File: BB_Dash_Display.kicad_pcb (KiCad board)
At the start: 2 copper layers, 54.6 x 61 mm, 47 parts, among them J1 FH12-40S-0.5SH, J2 Mini_SPOX, J3 Mini_SPOX, P8 BeagleBone_Black_Header, P9 BeagleBone_Black_Header, U1 TPS61165, U2 TCAN1042V, U3 TPS562200

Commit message: archive stuff
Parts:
- C1, C10, C11, C4, C5, C6, C7: footprint Capacitor_SMD:C_0805_2012Metric -> archive:C_0805_2012Metric
- C2, C8, C9: footprint Capacitor_SMD:C_1206_3216Metric -> archive:C_1206_3216Metric
- C3: footprint Capacitor_SMD:C_1210_3225Metric -> archive:C_1210_3225Metric
- D1, D2: footprint Diode_SMD:D_SOD-123 -> archive:D_SOD-123
- F1: footprint Fuse:Fuseholder_Littelfuse_Nano2_154x -> archive:Fuseholder_Littelfuse_Nano2_154x
- G***: footprint project:OUR-Logo -> archive:OUR-Logo
- J1: footprint Connector_FFC-FPC:Hirose_FH12-40S-0.5SH_1x40-1MP_P0.50mm_Horizontal -> archive:Hirose_FH12-40S-0.5SH_1x40-1MP_P0.50mm_Horizontal
- J2: footprint Connector_Molex:Molex_SPOX_5268-03A_1x03_P2.50mm_Horizontal -> archive:Molex_SPOX_5268-03A_1x03_P2.50mm_Horizontal
- J3: footprint Connector_Molex:Molex_SPOX_5268-02A_1x02_P2.50mm_Horizontal -> archive:Molex_SPOX_5268-02A_1x02_P2.50mm_Horizontal
- JP1: footprint Jumper:SolderJumper-2_P1.3mm_Open_TrianglePad1.0x1.5mm -> archive:SolderJumper-2_P1.3mm_Open_TrianglePad1.0x1.5mm
- L1, L2: footprint Inductor_SMD:L_Bourns-SRN4018 -> archive:L_Bourns-SRN4018
- P8, P9: footprint project:PinHeader_2x23_P2.54mm_Vertical_Flip -> archive:PinHeader_2x23_P2.54mm_Vertical_Flip
- R1, R2, R3, R4, R5, R6: footprint Resistor_SMD:R_0805_2012Metric -> archive:R_0805_2012Metric
- REF**: footprint project:BeagleBone-Black_Flip -> archive:BeagleBone-Black_Flip
- RN1, RN2, RN3, RN4, RN5: footprint Resistor_SMD:R_Array_Convex_4x0603 -> archive:R_Array_Convex_4x0603
- TP1, TP2, TP3, TP4, TP5, TP6, TP7, TP8, TP9: footprint TestPoint:TestPoint_THTPad_D2.0mm_Drill1.0mm -> archive:TestPoint_THTPad_D2.0mm_Drill1.0mm
- U1, U3: footprint Package_TO_SOT_SMD:SOT-23-6 -> archive:SOT-23-6
- U2: footprint Package_SO:SOIC-8_3.9x4.9mm_P1.27mm -> archive:SOIC-8_3.9x4.9mm_P1.27mm

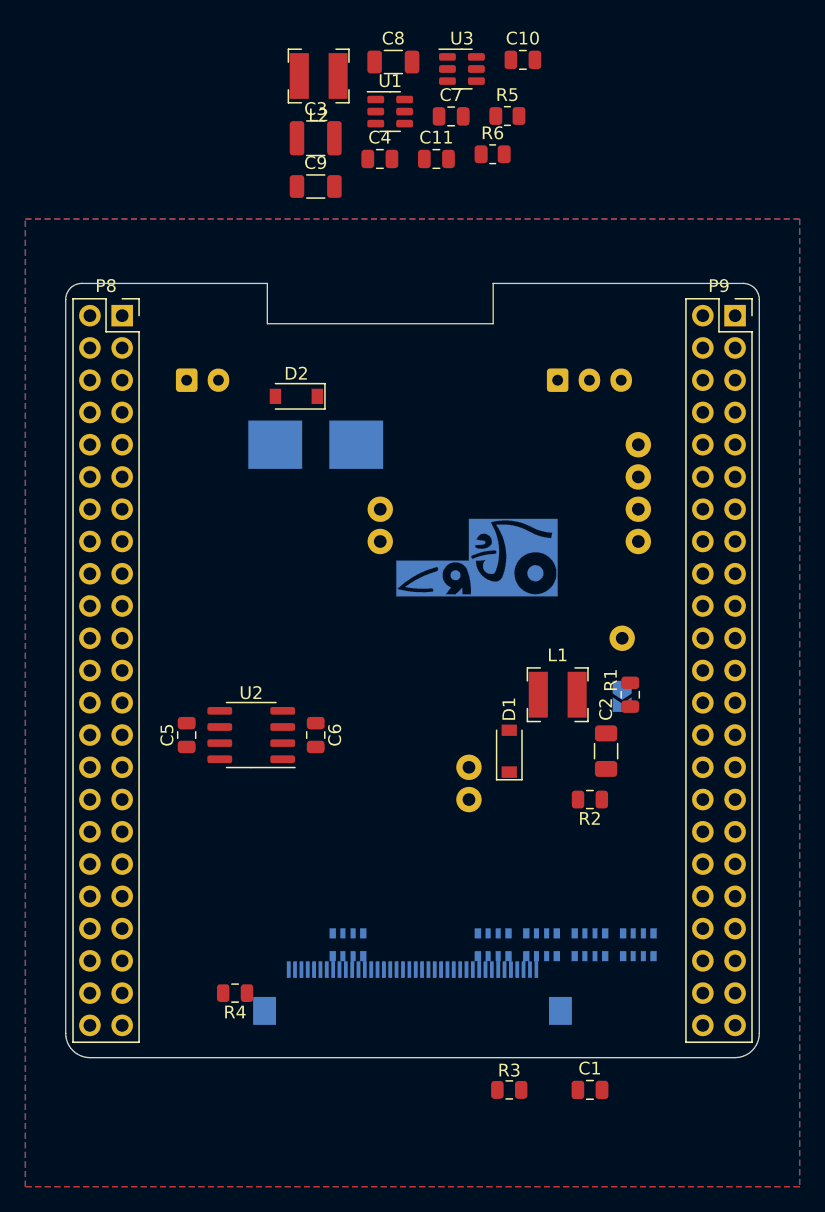
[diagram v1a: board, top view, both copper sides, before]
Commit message: rev b
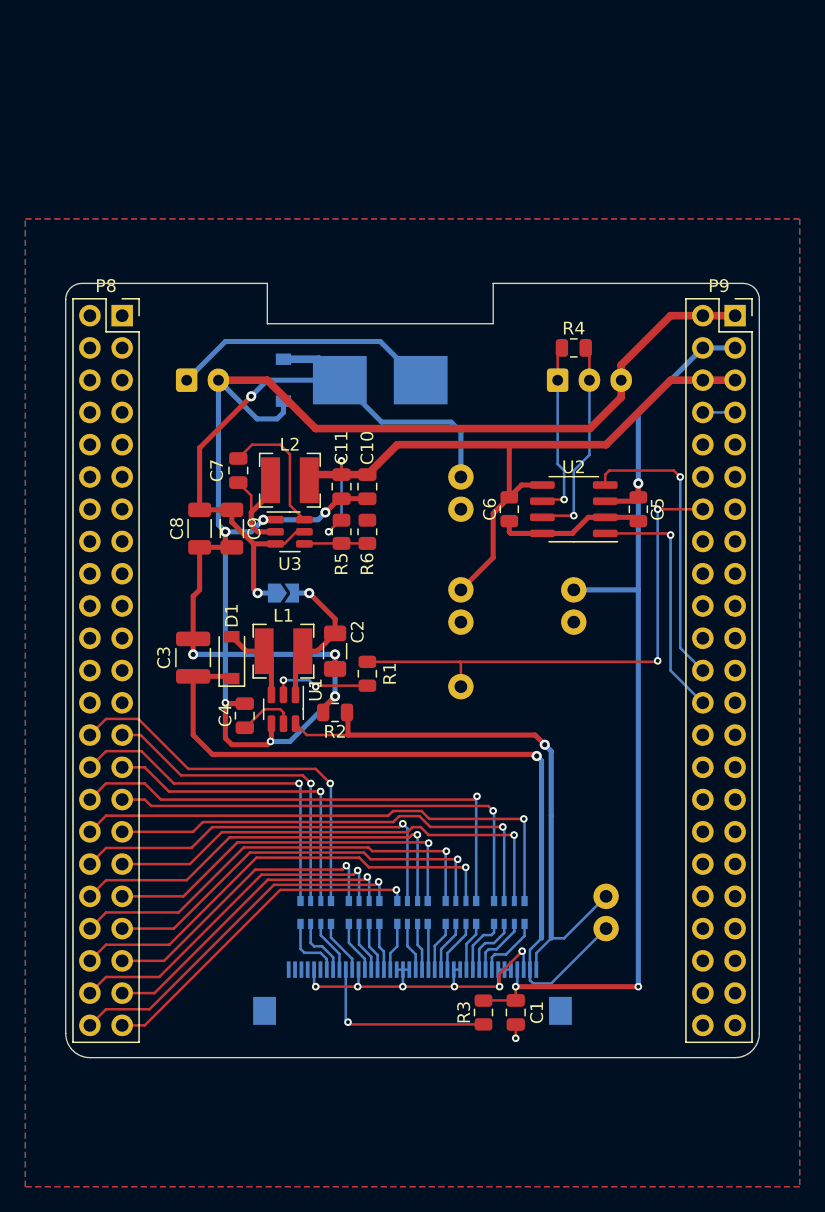
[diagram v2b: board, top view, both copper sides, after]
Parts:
- removed G***: LOGO, archive:OUR-Logo
- D2: moved to B.Cu
- moved R4 57.4 mm to (114.3, 78.7), turned to 180 degrees
- moved U1 47.8 mm to (91.4, 107.2), turned to 270 degrees
- moved C4 45.1 mm to (88.4, 107.7), turned to 90 degrees
- moved C3 42.0 mm to (84.3, 103.1), turned to 90 degrees
- moved C8 39.8 mm to (84.8, 93.0), turned to 270 degrees
- moved C5 39.8 mm to (119.4, 91.4)
- moved U3 38.9 mm to (91.9, 93.2)
- moved C10 35.8 mm to (98.0, 89.7), turned to 270 degrees
- moved R5 35.2 mm to (96.0, 93.2), turned to 270 degrees
- moved C7 32.5 mm to (87.9, 88.4), turned to 90 degrees
- moved L2 31.9 mm to (91.9, 89.2)
- moved R6 31.3 mm to (98.0, 93.2), turned to 90 degrees
- moved U2 31.0 mm to (114.3, 91.4)
- moved JP1 27.9 mm to (91.4, 98.0), turned to 0 degrees
- moved C9 27.7 mm to (87.4, 93.0), turned to 270 degrees
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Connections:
- J1 pad MP: GND -> Net-(J1-PadMP)
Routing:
- net GND: track 0.00 -> 182.8 mm, vias 0 -> 15
- net +3V3: track 0.00 -> 78.5 mm, vias 0 -> 3
- net /LED+: track 0.00 -> 61.6 mm, vias 0 -> 1
- net +5V: track 0.00 -> 61.3 mm, vias 0 -> 2
- net /V_IN: track 0.00 -> 53.7 mm, vias 0 -> 2
- net /LED-: track 0.00 -> 46.2 mm, vias 0 -> 1
- net /LCD_D11: track 0.00 -> 41.6 mm, vias 0 -> 1
- net /EHRPWM1A: track 0.00 -> 40.4 mm, vias 0 -> 2
- net /LCD_D15: track 0.00 -> 39.9 mm, vias 0 -> 1
- net /LCD_D12: track 0.00 -> 37.5 mm, vias 0 -> 1
- net /LCD_D13: track 0.00 -> 36.7 mm, vias 0 -> 1
- net /LCD_D14: track 0.00 -> 36.7 mm, vias 0 -> 1
- net /LCD_D5: track 0.00 -> 35.9 mm, vias 0 -> 1
- net /LCD_D7: track 0.00 -> 34.8 mm, vias 0 -> 1
- net /LCD_D9: track 0.00 -> 33.0 mm, vias 0 -> 1
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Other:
- net class Default: clearance 0.1524 -> 0.2; trace_width 0.1524 -> 0.2
- rule trace_clearance: 0.1524 -> 0.2
- board text added: "BL+"
- board text added: "BL-"
- board text added: "Dashboard Display BeagleBone CAN & LCD Version: Rev B Designed by: Andrew Chen Date: 2020-06-02"
- board text added: "VIN"
- board text removed: "CAN Termination"
- board text removed: "Dashboard Display BeagleBone CAN & LCD Version: Rev A3 Designed by: Andrew Chen Date: 2020-03-07"
- board text removed: "LED+"
- board text removed: "LED-"
- board text removed: "Vin"
